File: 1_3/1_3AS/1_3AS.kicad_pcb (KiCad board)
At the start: 2 copper layers, 118.5 x 93.4 mm, 45 parts, among them SW10 SW_SPST, SW11 SW_SPST, SW12 SW_SPST, SW14 SW_SPST, SW15 SW_SPST, SW16 SW_SPST, SW17 SW_SPST, SW18 SW_SPST, SW19 SW_SPST, SW2 SW_SPST, SW20 SW_SPST, SW21 SW_SPST, SW3 SW_SPST, SW4 SW_SPST, SW5 SW_SPST, SW6 SW_SPST, SW8 SW_SPST, SW9 SW_SPST, U1 XIAO_nRF52840

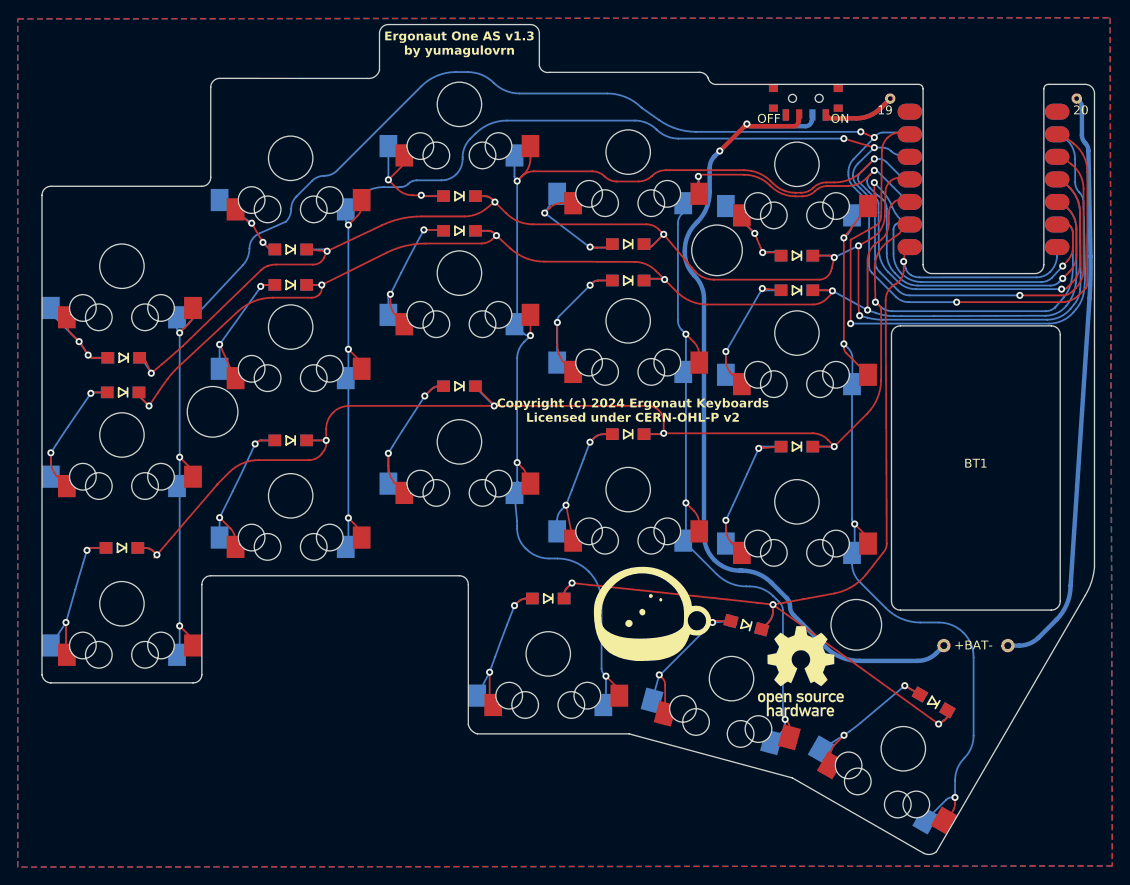
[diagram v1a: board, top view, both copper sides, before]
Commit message: 1_3AS chk
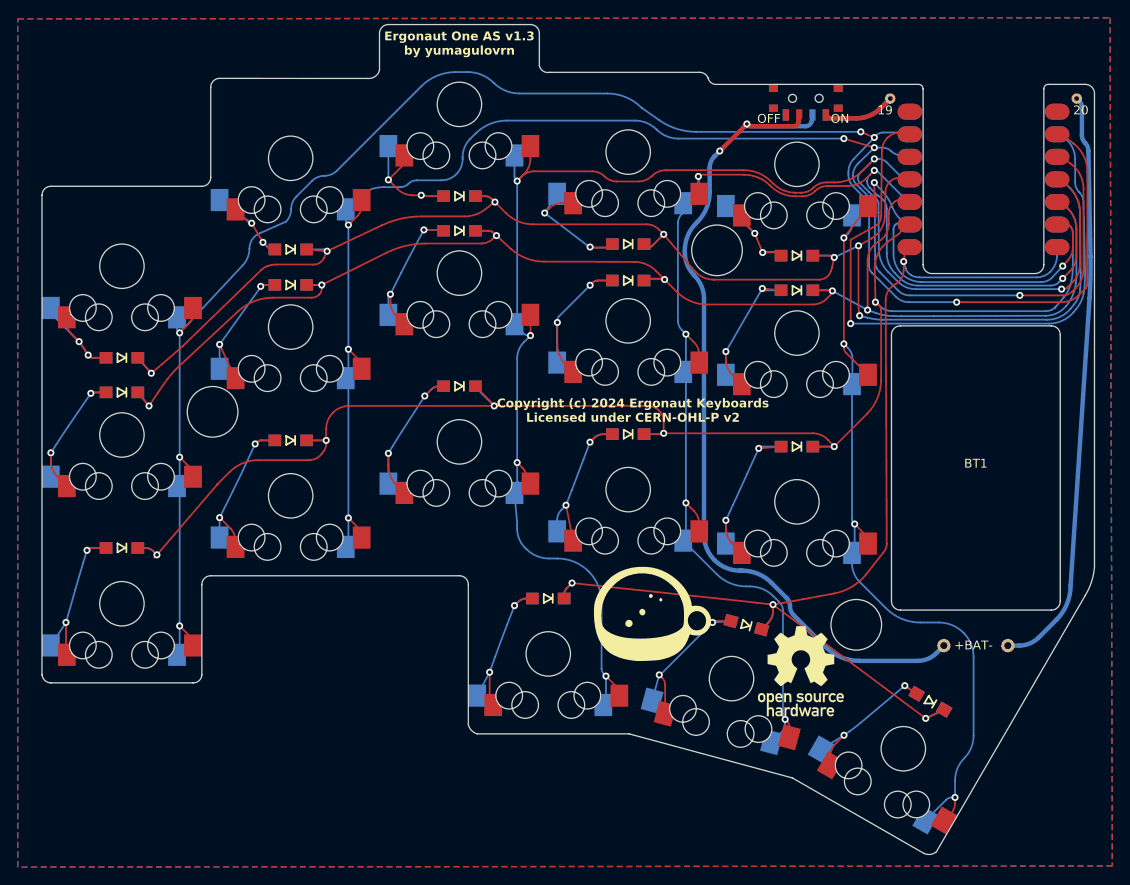
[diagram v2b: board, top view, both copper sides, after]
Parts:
- moved D21 0.38 mm to (194.5, 125.1)
- moved D2 0.20 mm to (103.5, 86.4)
- moved D8 0.13 mm to (103.5, 90.3)
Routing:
- net R1: track 162.6 -> 163.4 mm
- net Net-(D21-A): track 18.9 -> 18.1 mm
